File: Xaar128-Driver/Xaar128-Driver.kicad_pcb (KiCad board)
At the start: 2 copper layers, 171.7 x 157.5 mm, 172 parts, among them J1 Screw_Terminal_01x02, J3 Screw_Terminal_01x02, J4 Screw_Terminal_01x02, J5 Conn_01x21, J6 Conn_02x08_Odd_Even, J7 Screw_Terminal_01x04, Q1 DMN2075U, Q10 DMN2075U, Q11 DMG2305UX, Q2 DMN2075U, Q3 DMN2075U, Q4 DMN2075U, Q5 DMN2075U, Q6 DMN2075U, Q7 DMG2305UX, Q8 DMG2305UX, Q9 DMN2075U, U1 6N135, U10 74AHCT125, U11 LM317_TO-220, U12 TXB0104D, U13 MCP4725xxx-xCH, U14 ISO1540, U15 L7824, U16 MC78L05_SOT89, U18 MCP3021, U19 LTV-356T, U2 6N135, U20 74AHCT125, U21 74HC173, U3 74HC173, U4 NUCLEO-H743ZI2, U5 TXB0104D, U6 TXB0104D, U7 TXB0104D, U8 74AHCT125, U9 74AHCT125

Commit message: xaar driver: some routed islands
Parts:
- removed NT5: NetTie_2, NetTie:NetTie-2_SMD_Pad0.5mm
- added HS1: Heatsink, Xaar-Driver:SK68-375-SA, F.Cu at (51.8, 28.7)
- added U17: TLC272, Package_DIP:DIP-8_W7.62mm, F.Cu at (45.0, 77.5)
- JP10, JP11, JP12, JP13, JP15, JP16, JP3, JP8, JP9: footprint Resistor_SMD:R_0603_1608Metric -> Resistor_SMD:R_0603_1608Metric_Pad0.98x0.95mm_HandSolder
- NT1, NT3, NT4: moved to B.Cu
- moved JP16 308.8 mm to (-113.4, 48.3), turned to 0 degrees
- moved J5 306.1 mm to (-36.3, 161.2), turned to 180 degrees
- moved J4 303.1 mm to (358.1, 273.9)
- moved JP12 302.1 mm to (-113.4, 67.3)
- moved JP15 301.5 mm to (-113.4, 77.5)
- moved U6 300.9 mm to (-61.3, 148.8), turned to -90 degrees
- moved JP11 297.9 mm to (-113.4, 55.9), turned to 0 degrees
- moved JP9 296.4 mm to (-102.5, 53.1), turned to 0 degrees
- moved JP10 296.3 mm to (-113.4, 53.3), turned to 0 degrees
- moved JP8 295.8 mm to (-102.5, 48.3), turned to 0 degrees
- moved U4 293.6 mm to (-132.1, 26.8)
- moved JP13 288.8 mm to (-113.4, 58.4), turned to 0 degrees
- moved C9 282.1 mm to (-66.8, 152.1), turned to 90 degrees
- moved R18 281.8 mm to (-110.8, 33.8), turned to 90 degrees
- moved U10 278.7 mm to (-38.5, 149.0), turned to 90 degrees
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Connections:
- C13 pad 2: GNDHP -> GND1
- C14 pad 2: GNDHP -> GND1
- C16 pad 2: GNDHP -> GND1
- C17 pad 2: GNDHP -> GND1
- C19 pad 2: GNDHP -> GND1
- C20 pad 2: GND5HV -> GND1
- C21 pad 2: GND5HV -> GND1
- C23 pad 1: GND5HV -> GND1
- C25 pad 2: GND5HV -> GND1
- C26 pad 2: GND5HV -> GND1
- J3 pad 2: GNDHP -> GND1
- J5 pad 2: GNDHP -> GND1
- J5 pad 4: GNDHP -> GND1
- J6 pad 2: GNDHP -> GND1
- J6 pad 5: GNDHP -> GND1
- NT3 pad 1: GND5HV -> Net-(U15-IN)
- NT3 pad 2: GNDHP -> +36V
- NT4 pad 1: GNDHP -> +36V
- NT4 pad 2: GND24 -> Net-(NT4-Pad2)
- R1 pad 1: +36V -> Net-(NT4-Pad2)
- R40 pad 1: GND24 -> GND1
- R42 pad 2: GND5HV -> GND1
- R9 pad 1: +36V -> Net-(NT4-Pad2)
- U10 pad 11: /Level Shift/READY_OUT -> /Level Shift/nFAULT_OUT
- U10 pad 12: /Level Shift/READY_IN -> /Level Shift/nFAULT_IN
- U10 pad 2: /Level Shift/nFAULT_IN -> /Level Shift/nRESET_FAULT_IN
- U10 pad 3: /Level Shift/nFAULT_OUT -> /Level Shift/nRESET_FAULT_OUT
- U10 pad 8: /Level Shift/nRESET_FAULT_OUT -> /Level Shift/READY_OUT
- U10 pad 9: /Level Shift/nRESET_FAULT_IN -> /Level Shift/READY_IN
- U13 pad 2: GND5HV -> GND1
- U14 pad 5: GND5HV -> GND1
- U15 pad 1: +36V -> Net-(U15-IN)
- U15 pad 2: GND24 -> GND1
- U16 pad 2: GND5HV -> GND1
- U18 pad 1: (no net) -> +5VP
- U18 pad 2: (no net) -> GND1
- U18 pad 3: (no net) -> Net-(U18-AIN)
- U18 pad 4: (no net) -> SDA_HV
- U18 pad 5: (no net) -> SCL_HV
- U20 pad 11: unconnected-(U20-4Y-Pad11) -> /HV Supply/VPP_ENABLE_CP_5
- U20 pad 12: unconnected-(U20-4A-Pad12) -> /Level Shift/VPP_EN_CP_IN
- U20 pad 5: /Level Shift/VPP_EN_CP_IN -> unconnected-(U20-2A-Pad5)
- U20 pad 6: /HV Supply/VPP_ENABLE_CP_5 -> unconnected-(U20-2Y-Pad6)
- U5 pad 12: /Level Shift/nSS2_OUT -> /Level Shift/nSS1_OUT
- U5 pad 13: /Level Shift/nSS1_OUT -> /Level Shift/PHO_OUT
- U5 pad 2: /Level Shift/nSS1_IN -> /Level Shift/PHO_IN
- U5 pad 3: /Level Shift/nSS2_IN -> /Level Shift/nSS1_IN
- U6 pad 10: /Level Shift/RESET_DISABLE_CP_OUT -> unconnected-(U6-B4-Pad10)
- U6 pad 11: /Level Shift/PHO_OUT -> /IO/nFIRE
- U6 pad 12: /IO/nFIRE -> /Level Shift/CLK_OUT
- U6 pad 13: /Level Shift/CLK_OUT -> /Level Shift/nSS2_OUT
- U6 pad 2: /Level Shift/CLK_IN -> /Level Shift/nSS2_IN
- U6 pad 3: /Level Shift/nFIRE_IN -> /Level Shift/CLK_IN
- U6 pad 4: /Level Shift/PHO_IN -> /Level Shift/nFIRE_IN
- U6 pad 5: /Level Shift/RESET_DISABLE_CP_IN -> unconnected-(U6-A4-Pad5)
- U7 pad 10: /Level Shift/nRESET_FAULT_OUT -> /Level Shift/READY_OUT
- U7 pad 12: /Level Shift/READY_OUT -> /Level Shift/nFAULT_OUT
- U7 pad 13: /Level Shift/nFAULT_OUT -> /Level Shift/nRESET_FAULT_OUT
- U7 pad 2: /Level Shift/nFAULT_IN -> /Level Shift/nRESET_FAULT_IN
- U7 pad 3: /Level Shift/READY_IN -> /Level Shift/nFAULT_IN
- U7 pad 5: /Level Shift/nRESET_FAULT_IN -> /Level Shift/READY_IN
- U8 pad 11: /Level Shift/MOSI_OUT -> /Level Shift/nSS1_OUT
- U8 pad 12: /Level Shift/MOSI_IN -> /Level Shift/nSS1_IN
- U8 pad 2: /Level Shift/nSS1_IN -> /Level Shift/PHO_IN
- U8 pad 3: /Level Shift/nSS1_OUT -> /Level Shift/PHO_OUT
- U8 pad 5: /Level Shift/nSS2_IN -> /Level Shift/SCK_IN
- U8 pad 6: /Level Shift/nSS2_OUT -> /Level Shift/SCK_OUT
- U8 pad 8: /Level Shift/SCK_OUT -> /Level Shift/MOSI_OUT
- U8 pad 9: /Level Shift/SCK_IN -> /Level Shift/MOSI_IN
- U9 pad 11: unconnected-(U9-4Y-Pad11) -> /Level Shift/CLK_OUT
- U9 pad 12: unconnected-(U9-4A-Pad12) -> /Level Shift/CLK_IN
- U9 pad 2: /Level Shift/CLK_IN -> /Level Shift/nSS2_IN
- U9 pad 3: /Level Shift/CLK_OUT -> /Level Shift/nSS2_OUT
- U9 pad 8: /Level Shift/PHO_OUT -> unconnected-(U9-3Y-Pad8)
- U9 pad 9: /Level Shift/PHO_IN -> unconnected-(U9-3A-Pad9)
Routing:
- net GND1: track 0.00 -> 167.8 mm
- net GND: track 0.00 -> 137.6 mm, vias 0 -> 18
- net +5V: track 0.00 -> 106.8 mm, vias 0 -> 6
- net +3.3V: track 0.00 -> 75.9 mm, vias 0 -> 3
- net /Level Shift/nRESET_IN: track 16.7 -> 63.2 mm
- net /Level Shift/nSS2_OUT: track 0.00 -> 40.4 mm, vias 0 -> 2
- net /Level Shift/SCK_OUT: track 0.00 -> 38.2 mm, vias 0 -> 2
- net /IO/nFIRE: track 8.59 -> 44.2 mm
- net OE_OUT: track 0.00 -> 34.3 mm, vias 0 -> 2
- net /Level Shift/MOSI_OUT: track 0.00 -> 33.9 mm, vias 0 -> 2
- net Net-(U15-IN): track 0.00 -> 33.1 mm
- net /Level Shift/nSS1_OUT: track 0.00 -> 32.2 mm, vias 0 -> 2
- net /Level Shift/PHO_OUT: track 3.11 -> 35.1 mm, vias 0 -> 2
- net /Level Shift/CLK_OUT: track 8.59 -> 37.6 mm
- net ~{OE_OUT}: track 14.8 -> 43.0 mm
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- added copper zone on F.Cu, net GND
- added copper zone on F.Cu, net GND1
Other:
- board size 171.7 x 157.5 mm -> 528.8 x 460 mm

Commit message: xaar driver pcb: order elements
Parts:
- moved C27 641.7 mm to (-245.3, 23.8)
- moved J1 641.7 mm to (-304.3, 29.2)
- moved J7 641.7 mm to (-283.7, 29.5)
- moved NT2 641.7 mm to (-294.1, 18.8)
- moved NT6 641.7 mm to (-265.4, 13.9)
- moved NT7 641.7 mm to (-276.1, 15.4)
- moved Q9 641.7 mm to (-240.0, 29.1)
- moved R43 641.7 mm to (-241.0, 21.1)
- moved J4 641.7 mm to (-247.4, 61.5)
- moved R14 420.6 mm to (-150.6, 198.0)
- moved R15 420.6 mm to (-150.6, 199.5)
- moved R45 420.6 mm to (-149.6, 191.9)
- moved R49 420.6 mm to (-151.1, 193.7)
- moved U3 420.6 mm to (-145.0, 194.9)
- moved C7 420.6 mm to (-147.8, 188.1)
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
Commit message: more components routed
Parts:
- moved R59 186.5 mm to (-4.32, 88.9)
- moved R29 182.8 mm to (-5.33, 94.7)
- moved R27 180.1 mm to (19.9, 91.8), turned to 90 degrees
- moved D9 179.5 mm to (22.5, 88.8), turned to -90 degrees
- moved TP5 177.7 mm to (19.6, 96.3), turned to 90 degrees
- moved R28 176.5 mm to (22.5, 92.6), turned to -90 degrees
- moved JP14 174.4 mm to (1.78, 92.9), turned to 180 degrees
- moved U19 173.9 mm to (14.4, 89.0), turned to 0 degrees
- moved TP10 168.3 mm to (20.1, 85.9)
- moved Q7 167.2 mm to (23.1, 100.1), turned to 180 degrees
- moved Q8 164.8 mm to (30.1, 100.2), turned to -90 degrees
- moved C11 162.5 mm to (28.4, 89.7), turned to 90 degrees
- moved C14 161.7 mm to (57.1, 98.8), turned to 90 degrees
- moved C12 160.1 mm to (26.7, 94.7), turned to -90 degrees
- moved C16 154.6 mm to (40.2, 96.2), turned to 90 degrees
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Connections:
- U4 pad 12: /Level Shift/READY_OUT -> /Level Shift/nRESET_OUT
- U4 pad 14: /Level Shift/nRESET_FAULT_OUT -> /Level Shift/READY_OUT
- U4 pad 9: /Level Shift/nRESET_OUT -> /Level Shift/nRESET_FAULT_OUT
- U4 pad CN7_1: Net-(JP3-B) -> /Level Shift/COMM_ENABLE
- U4 pad CN7_3: /Level Shift/COMM_ENABLE -> Net-(JP3-B)
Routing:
- net GND: track 137.6 -> 266.2 mm, vias 18 -> 24
- net GND1: track 167.8 -> 246.4 mm, vias 0 -> 2
- net /Level Shift/SCK_IN: track 13.4 -> 70.6 mm
- net /MCU/SCL: track 0.00 -> 56.2 mm
- net /Level Shift/CLK_IN: track 18.6 -> 73.4 mm
- net /MCU/SDA: track 0.00 -> 52.7 mm
- net /Level Shift/nSS1_IN: track 17.6 -> 70.0 mm, vias 2 -> 4
- net /Level Shift/READY_OUT: track 16.4 -> 64.7 mm
- net /Level Shift/nFAULT_OUT: track 15.8 -> 63.9 mm, vias 2 -> 5
- net /Level Shift/MOSI_IN: track 16.4 -> 64.1 mm
- net /Level Shift/nRESET_OUT: track 21.5 -> 65.1 mm
- net /Level Shift/nFIRE_IN: track 15.4 -> 58.7 mm, vias 2 -> 3
- net Net-(D7-K): track 0.22 -> 39.9 mm, vias 0 -> 1
- net /Level Shift/nSS2_IN: track 16.5 -> 51.5 mm, vias 2 -> 3
- net /Level Shift/nRESET_FAULT_OUT: track 19.9 -> 54.9 mm
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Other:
- board size 528.8 x 460 mm -> 270.9 x 235.8 mm

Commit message: more routing
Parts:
- removed NT4: NetTie_2, NetTie:NetTie-2_SMD_Pad0.5mm
- removed R48: 100k, Resistor_SMD:R_0603_1608Metric_Pad0.98x0.95mm_HandSolder
- moved TP13 135.6 mm to (-42.4, 94.5), turned to 180 degrees
- moved C30 131.4 mm to (-16.8, 117.6), turned to 90 degrees
- moved C31 129.3 mm to (-48.3, 100.1)
- moved C28 125.7 mm to (-16.8, 121.9)
- moved R19 125.5 mm to (-24.9, 115.1)
- moved R52 124.6 mm to (-40.0, 99.3), turned to 90 degrees
- moved U12 124.6 mm to (-22.1, 119.6), turned to 90 degrees
- moved HS1 122.0 mm to (76.0, 148.3), turned to -90 degrees
- moved C29 119.4 mm to (-16.8, 127.5), turned to 90 degrees
- moved R44 119.1 mm to (-44.7, 112.3), turned to 0 degrees
- moved R51 118.1 mm to (-38.1, 102.1), turned to 90 degrees
- moved Q4 116.3 mm to (-50.0, 103.4)
- moved R21 116.1 mm to (-47.2, 110.5), turned to -90 degrees
- moved U21 115.0 mm to (-42.7, 106.4)
- moved R50 114.6 mm to (-44.7, 100.3)
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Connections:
- U12 pad 12: /HV Supply/VPP_ENABLE_CP_5 -> /Level Shift/RESET_DISABLE_CP_OUT
- U12 pad 13: /Level Shift/RESET_DISABLE_CP_OUT -> /HV Supply/VPP_ENABLE_CP_5
- U12 pad 2: /Level Shift/RESET_DISABLE_CP_IN -> /Level Shift/VPP_EN_CP_IN
- U12 pad 3: /Level Shift/VPP_EN_CP_IN -> /Level Shift/RESET_DISABLE_CP_IN
- U20 pad 11: /HV Supply/VPP_ENABLE_CP_5 -> /Level Shift/RESET_DISABLE_CP_OUT
- U20 pad 12: /Level Shift/VPP_EN_CP_IN -> /Level Shift/RESET_DISABLE_CP_IN
- U20 pad 2: /Level Shift/RESET_DISABLE_CP_IN -> /Level Shift/VPP_EN_CP_IN
- U20 pad 3: /Level Shift/RESET_DISABLE_CP_OUT -> /HV Supply/VPP_ENABLE_CP_5
- U4 pad 11: /MCU/nRESET_MCU -> /Level Shift/VPP_EN_CP_IN
- U4 pad 13: /Level Shift/VPP_EN_CP_IN -> /MCU/nRESET_MCU
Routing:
- net GND: track 266.2 -> 420.8 mm, vias 24 -> 37
- net +5V: track 127.2 -> 226.6 mm, vias 6 -> 7
- net /Level Shift/nRESET_IN: track 62.1 -> 100.3 mm, vias 2 -> 6
- net /Level Shift/nRESET_FAULT_IN: track 16.5 -> 50.4 mm, vias 2 -> 5
- net Net-(JP14-B): track 0.00 -> 30.8 mm
- net /Level Shift/nFAULT_IN: track 27.3 -> 56.0 mm
- net /Level Shift/VPP_EN_CP_IN: track 17.6 -> 44.3 mm, vias 2 -> 3
- net Net-(JP14-C): track 0.00 -> 26.7 mm, vias 0 -> 1
- net /HV Supply/VPP_EN: track 28.8 -> 52.0 mm
- net /HV Supply/VPP_ENABLE_CP_5: track 15.8 -> 37.0 mm, vias 2 -> 4
- net Net-(JP14-A): track 0.00 -> 18.0 mm
- net /Level Shift/RESET_DISABLE_CP_IN: track 16.5 -> 34.1 mm
- net Net-(Q4-S): track 0.00 -> 16.9 mm
- net +36V: track 24.3 -> 10.4 mm
- net Net-(D9-A): track 14.5 -> 27.8 mm, vias 0 -> 2
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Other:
- board size 270.9 x 235.8 mm -> 216.7 x 184.3 mm

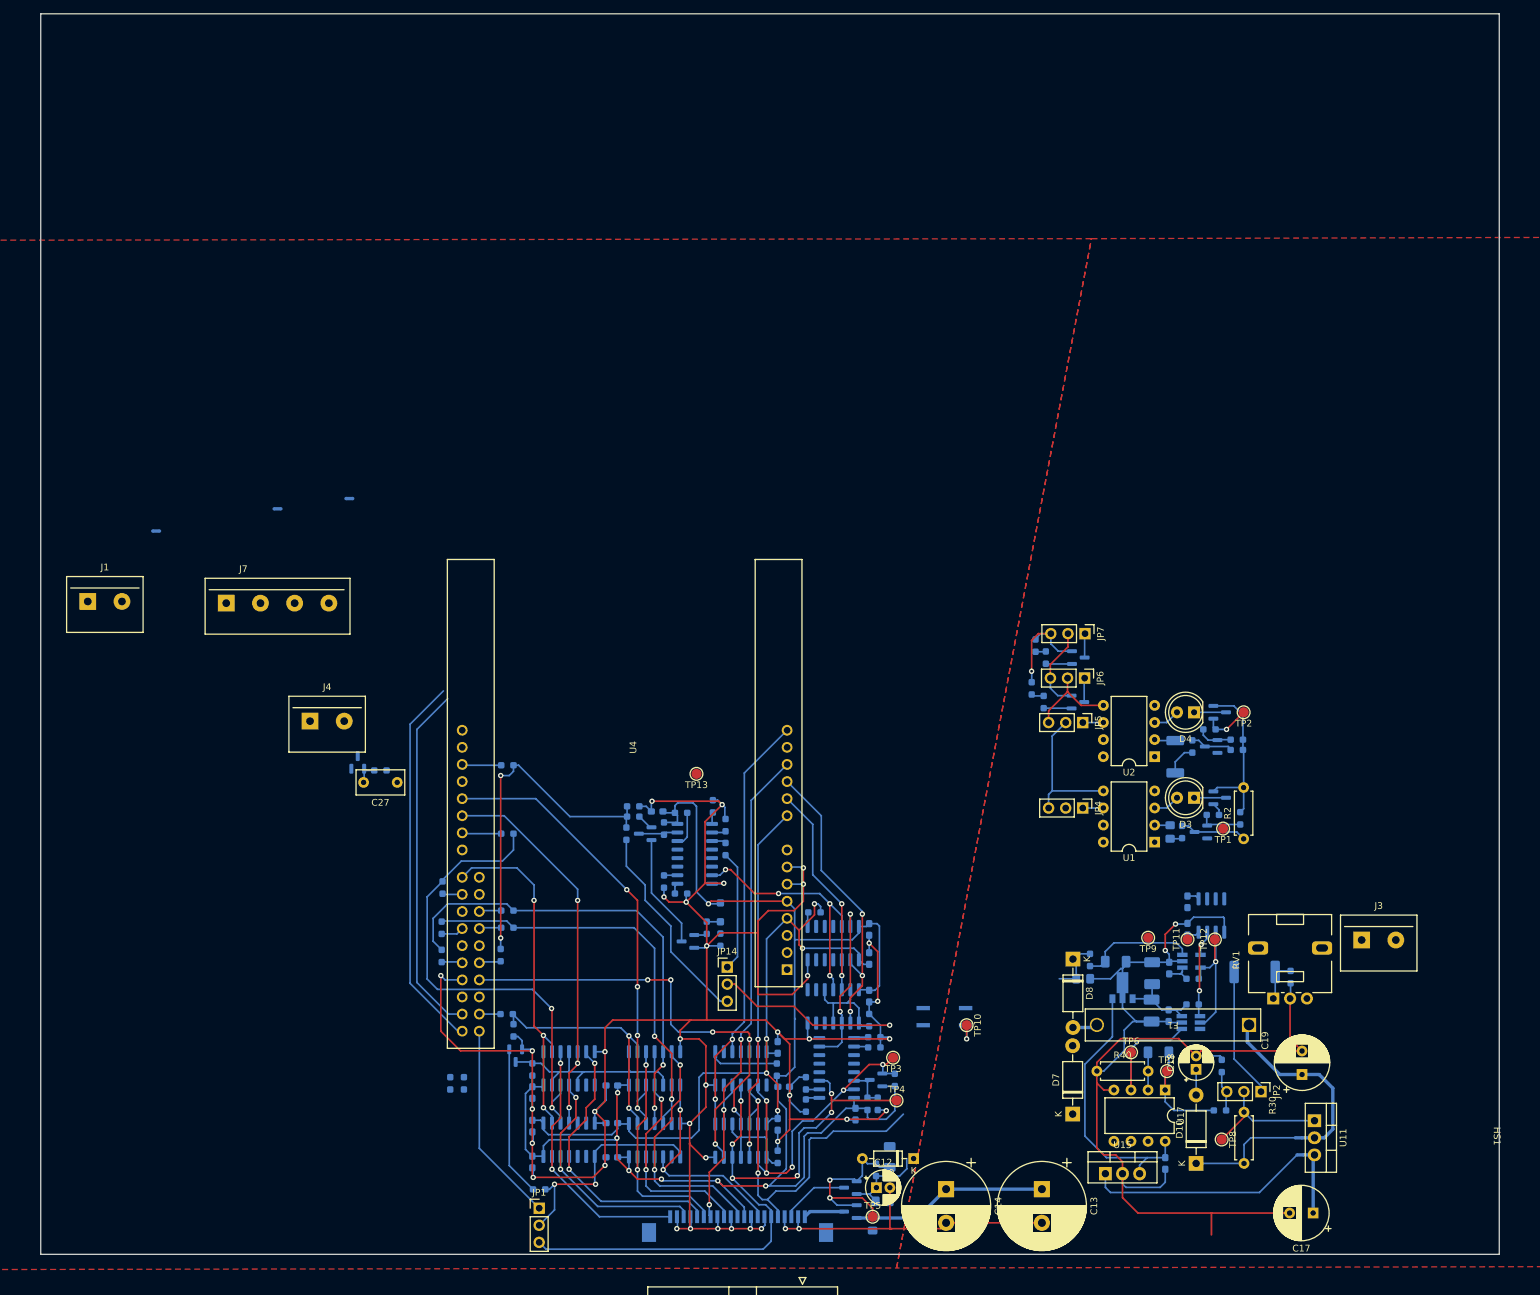
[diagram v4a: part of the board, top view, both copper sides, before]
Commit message: more routing
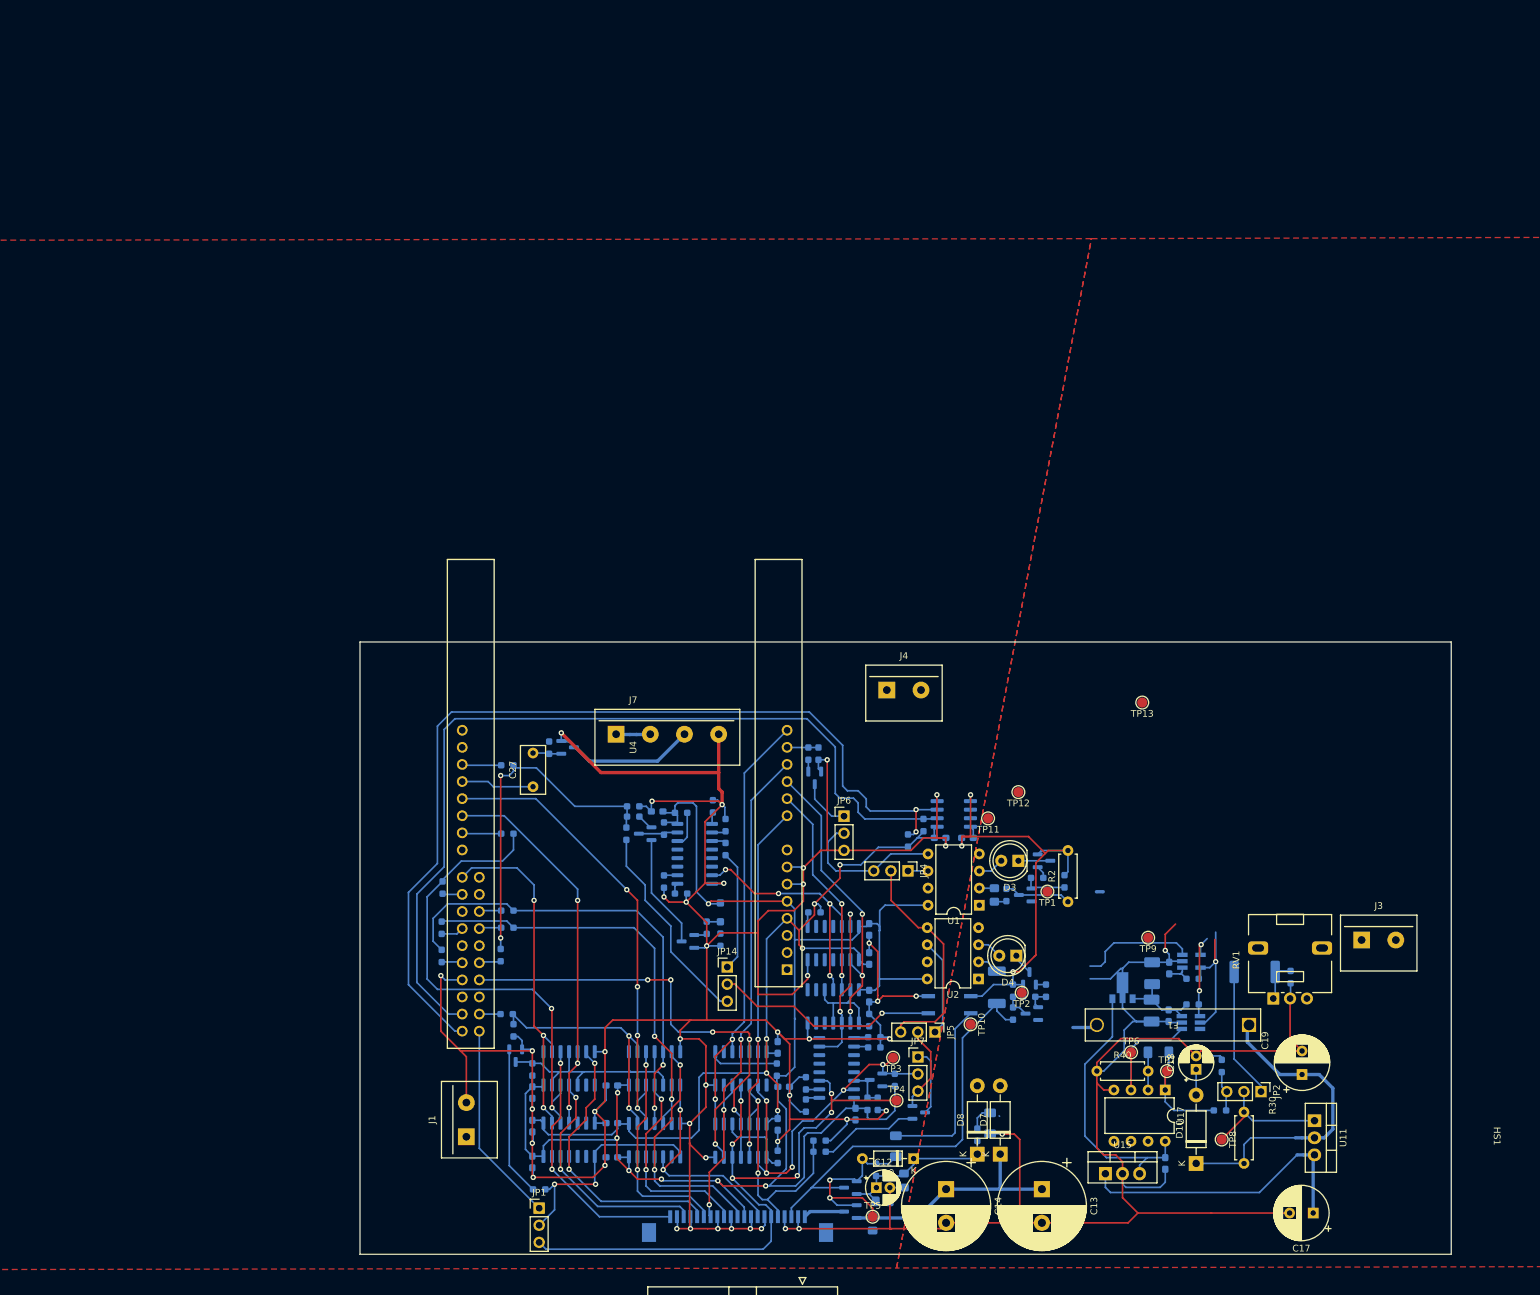
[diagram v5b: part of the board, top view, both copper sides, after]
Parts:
- removed NT2, NT6: NetTie_2, NetTie:NetTie-2_SMD_Pad0.5mm
- removed R47: 100k, Resistor_SMD:R_0603_1608Metric_Pad0.98x0.95mm_HandSolder
- added NT4: NetTie_2, NetTie:NetTie-2_SMD_Pad0.5mm, B.Cu at (17.5, 112.0)
- added R22: 1k, Resistor_SMD:R_0603_1608Metric_Pad0.98x0.95mm_HandSolder, B.Cu at (-24.1, 150.6)
- R46: value 1k -> 100k
- moved J1 97.4 mm to (-76.6, 148.4), turned to 90 degrees
- moved J4 85.8 mm to (-14.1, 82.0)
- moved R36 80.1 mm to (-8.70, 102.1), turned to 90 degrees
- moved R46 79.2 mm to (-24.1, 149.0), turned to 0 degrees
- moved R35 75.2 mm to (-11.0, 104.4), turned to 90 degrees
- moved Q10 71.6 mm to (-9.40, 144.8)
- moved JP7 67.6 mm to (-9.53, 136.5), turned to 0 degrees
- moved TP13 67.1 mm to (23.8, 83.9)
- moved NT7 62.6 mm to (-51.8, 88.6), turned to 0 degrees
- moved J7 61.1 mm to (-54.4, 88.6)
- moved TP2 53.1 mm to (5.90, 127.0)
- moved JP5 51.0 mm to (-7.00, 132.8)
- moved R6 49.1 mm to (7.00, 127.6), turned to 180 degrees
- moved R4 48.8 mm to (4.60, 126.7), turned to 90 degrees
- moved Q2 48.6 mm to (7.05, 124.9), turned to 90 degrees
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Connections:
- J7 pad 4: LEDPWRGND -> GND
- JP4 pad 2: /Level Shift/nRESET_FAULT_IN -> Net-(JP4-C)
- JP5 pad 2: Net-(JP4-B) -> Net-(JP5-C)
- JP5 pad 3: Net-(JP5-B) -> Net-(JP4-C)
- JP6 pad 2: Net-(JP5-B) -> Net-(JP4-B)
- JP6 pad 3: Net-(JP6-B) -> GND
- JP7 pad 2: Net-(JP6-B) -> /Level Shift/nRESET_FAULT_IN
- JP7 pad 3: GND -> Net-(JP5-C)
- Q10 pad 2: GND -> Net-(JP5-C)
- Q3 pad 2: Net-(JP6-B) -> GND
- Q9 pad 2: LEDPWRGND -> GND
- R43 pad 2: Net-(NT6-Pad1) -> GND
- R46 pad 2: Net-(Q10-G) -> GND
- U2 pad 5: Net-(JP5-B) -> Net-(JP4-C)
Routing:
- net GND: track 420.8 -> 513.4 mm, vias 37 -> 41
- net /MCU/SCL: track 56.2 -> 141.5 mm, vias 0 -> 2
- net /MCU/SDA: track 52.7 -> 132.9 mm
- net GND1: track 249.3 -> 313.2 mm, vias 4 -> 7
- net /HV Supply/VPPL: track 14.9 -> 62.2 mm
- net Net-(JP4-C): track 0.00 -> 33.3 mm
- net +3.3V: track 110.8 -> 135.2 mm, vias 5 -> 6
- net Net-(R27-Pad2): track 4.13 -> 27.7 mm, vias 1 -> 0
- net /IO/LED-: track 0.00 -> 18.9 mm
- net +5V: track 226.6 -> 244.2 mm
- net /Level Shift/nFAULT_IN: track 56.0 -> 38.8 mm
- net Net-(JP5-B): track 13.9 -> 0.00 mm
- net Net-(JP5-C): track 0.00 -> 12.9 mm
- net Net-(JP6-B): track 12.8 -> 0.00 mm
- net Net-(JP5-A): track 3.06 -> 14.4 mm
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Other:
- board size 216.7 x 184.3 mm -> 162.1 x 91 mm
